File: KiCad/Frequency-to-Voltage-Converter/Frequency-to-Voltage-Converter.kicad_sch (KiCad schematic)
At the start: 34 parts, among them J1 Conn_Coaxial, J2 Conn_Coaxial, U1 MC12093D, U2 MC12093D, U3 VFC110AP

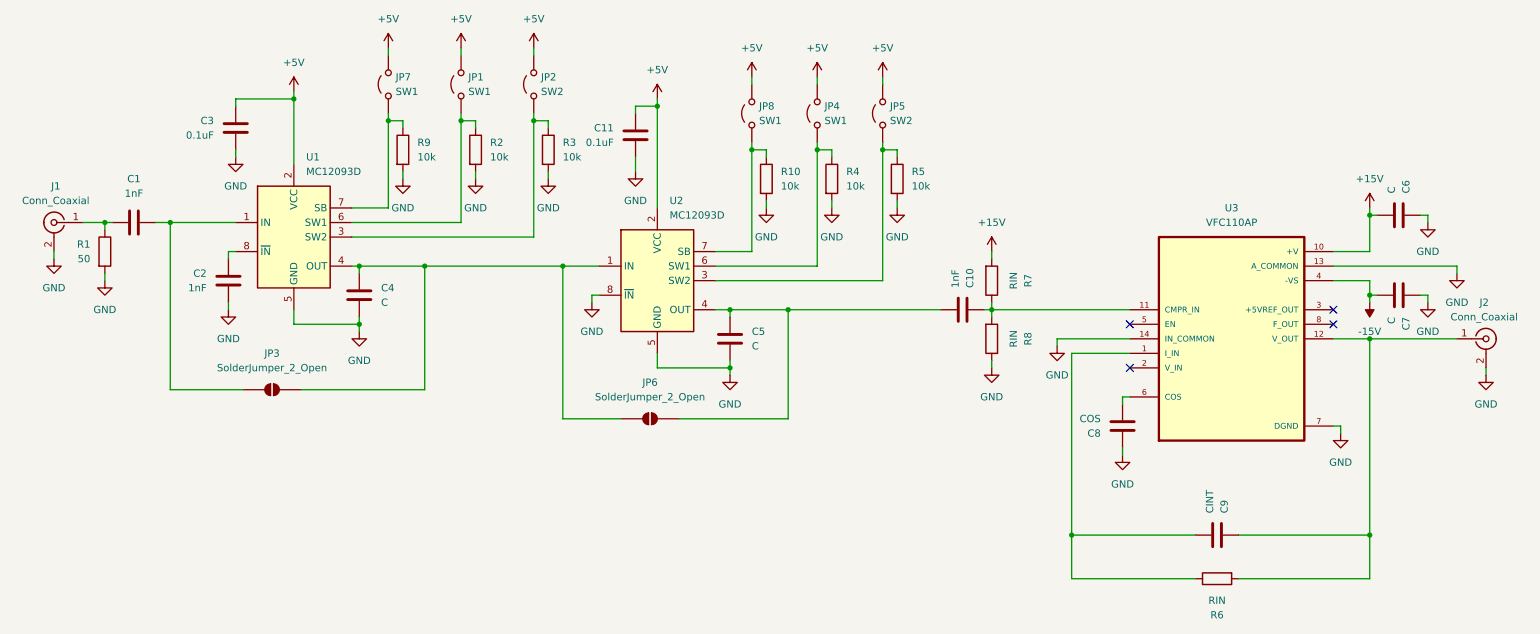
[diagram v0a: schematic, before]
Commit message: Updated schematic
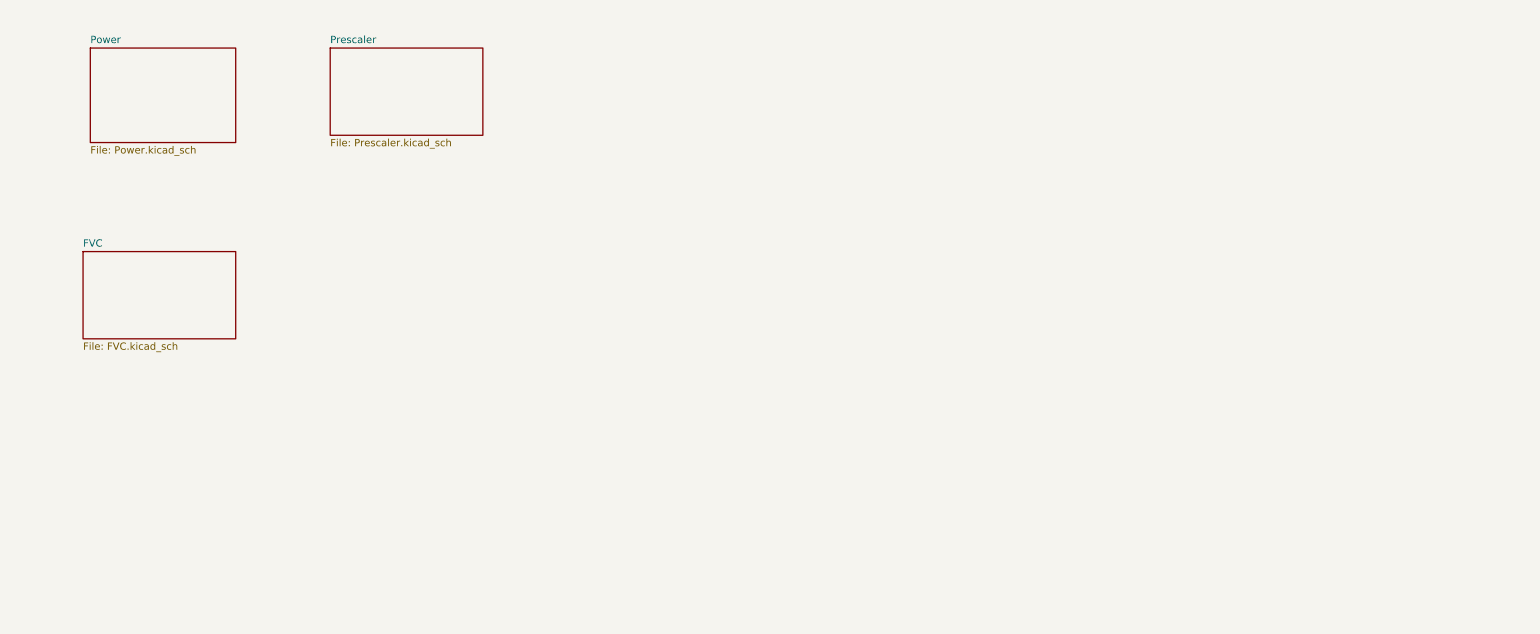
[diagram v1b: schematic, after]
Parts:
- removed C1, C10, C2: 1nF, symbol Device:C
- removed C11, C3: 0.1uF, symbol Device:C
- removed C4, C5, C6, C7: C, symbol Device:C
- removed C8: COS, symbol Device:C
- removed C9: CINT, symbol Device:C
- removed J1, J2: Conn_Coaxial, symbol Connector:Conn_Coaxial
- removed JP1, JP4, JP7, JP8: SW1, symbol Jumper:Jumper_2_Open
- removed JP2, JP5: SW2, symbol Jumper:Jumper_2_Open
- removed JP3, JP6: SolderJumper_2_Open, symbol Jumper:SolderJumper_2_Open
- removed R1: 50, symbol Device:R
- removed R10, R2, R3, R4, R5, R9: 10k, symbol Device:R
- removed R6, R7, R8: RIN, symbol Device:R
- removed U1, U2: MC12093D, Package_SO:SOIC-8_3.9x4.9mm_P1.27mm, symbol RF:MC12093D
- removed U3: VFC110AP, VFC110AP:DIP794W45P254L1969H508Q14, symbol VFC110AP:VFC110AP
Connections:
- no-connect marks 4 -> 0
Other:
- added sheet FVC (FVC.kicad_sch)
- added sheet Power (Power.kicad_sch)
- added sheet Prescaler (Prescaler.kicad_sch)
